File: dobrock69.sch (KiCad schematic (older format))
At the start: 159 parts, among them J1 HDMI_A_1.4, J2 Conn_01x02, J3 Conn_01x03, U1 XC6206P332MR, U2 STM32L072KBUx

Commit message: PCB switch daitai haichi shita
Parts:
- MX59, MX60, MX61, MX64, MX65, MX66: footprint kbd:CherryMX_Choc_Hotswap -> kbd:Choc_Hotswap
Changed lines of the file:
@@
 F 0 "MX60" H 3308 4298 60  0000 C CNN
 F 1 "MX-NoLED" H 3308 4224 20  0000 C CNN
-F 2 "kbd:CherryMX_Choc_Hotswap" H 2650 4050 60  0001 C CNN
+F 2 "kbd:Choc_Hotswap" H 2650 4050 60  0001 C CNN
 F 3 "" H 2650 4050 60  0001 C CNN
 	1    3275 4075
@@
 F 0 "MX59" H 2858 4298 60  0000 C CNN
 F 1 "MX-NoLED" H 2858 4224 20  0000 C CNN
-F 2 "kbd:CherryMX_Choc_Hotswap" H 2200 4050 60  0001 C CNN
+F 2 "kbd:Choc_Hotswap" H 2200 4050 60  0001 C CNN
 F 3 "" H 2200 4050 60  0001 C CNN
 	1    2825 4075
@@
 F 0 "MX61" H 3808 4298 60  0000 C CNN
 F 1 "MX-NoLED" H 3808 4224 20  0000 C CNN
-F 2 "kbd:CherryMX_Choc_Hotswap" H 3150 4050 60  0001 C CNN
+F 2 "kbd:Choc_Hotswap" H 3150 4050 60  0001 C CNN
 F 3 "" H 3150 4050 60  0001 C CNN
 	1    3775 4075
@@
 F 0 "MX64" H 9808 4373 60  0000 C CNN
 F 1 "MX-NoLED" H 9808 4299 20  0000 C CNN
-F 2 "kbd:CherryMX_Choc_Hotswap" H 9150 4125 60  0001 C CNN
+F 2 "kbd:Choc_Hotswap" H 9150 4125 60  0001 C CNN
 F 3 "" H 9150 4125 60  0001 C CNN
 	1    9775 4150
@@
 F 0 "MX66" H 10833 4373 60  0000 C CNN
 F 1 "MX-NoLED" H 10833 4299 20  0000 C CNN
-F 2 "kbd:CherryMX_Choc_Hotswap" H 10175 4125 60  0001 C CNN
+F 2 "kbd:Choc_Hotswap" H 10175 4125 60  0001 C CNN
 F 3 "" H 10175 4125 60  0001 C CNN
 	1    10800 4150
@@
 F 0 "MX65" H 10333 4373 60  0000 C CNN
 F 1 "MX-NoLED" H 10333 4299 20  0000 C CNN
-F 2 "kbd:CherryMX_Choc_Hotswap" H 9675 4125 60  0001 C CNN
+F 2 "kbd:Choc_Hotswap" H 9675 4125 60  0001 C CNN
 F 3 "" H 9675 4125 60  0001 C CNN
 	1    10300 4150

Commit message: pcb susunda
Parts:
- MX1, MX10, MX11, MX12, MX13, MX14, MX15, MX16, MX18, MX19, MX20, MX21, MX22, MX23, MX24, MX25, MX26, MX27, MX28, MX3, MX30, MX32, MX33, MX34, MX35, MX36, MX37, MX38, MX39, MX4, MX40, MX41, MX42, MX44, MX45, MX49, MX5, MX50, MX53, MX54, MX55, MX56, MX57, MX58, MX6, MX62, MX63, MX67, MX68, MX69, MX7, MX8, MX9: footprint MX_Only:MXOnly-1U-Hotswap -> MX_Only:MXOnly-1U-NoLED
- MX17, MX29: footprint MX_Only:MXOnly-1.75U-Hotswap -> MX_Only:MXOnly-1.75U-NoLED
- MX2: footprint MX_Only:MXOnly-1.5U-Hotswap -> MX_Only:MXOnly-1.5U-NoLED
- MX31, MX43, MX48, MX51: footprint MX_Only:MXOnly-2.25U-Hotswap -> MX_Only:MXOnly-2.25U-NoLED
- MX46, MX47, MX52: footprint MX_Only:MXOnly-1.25U-Hotswap -> MX_Only:MXOnly-1.25U-NoLED
- MX59, MX60, MX61, MX64, MX65, MX66: footprint kbd:Choc_Hotswap -> Kailh_Choc:KailhChoc-1U

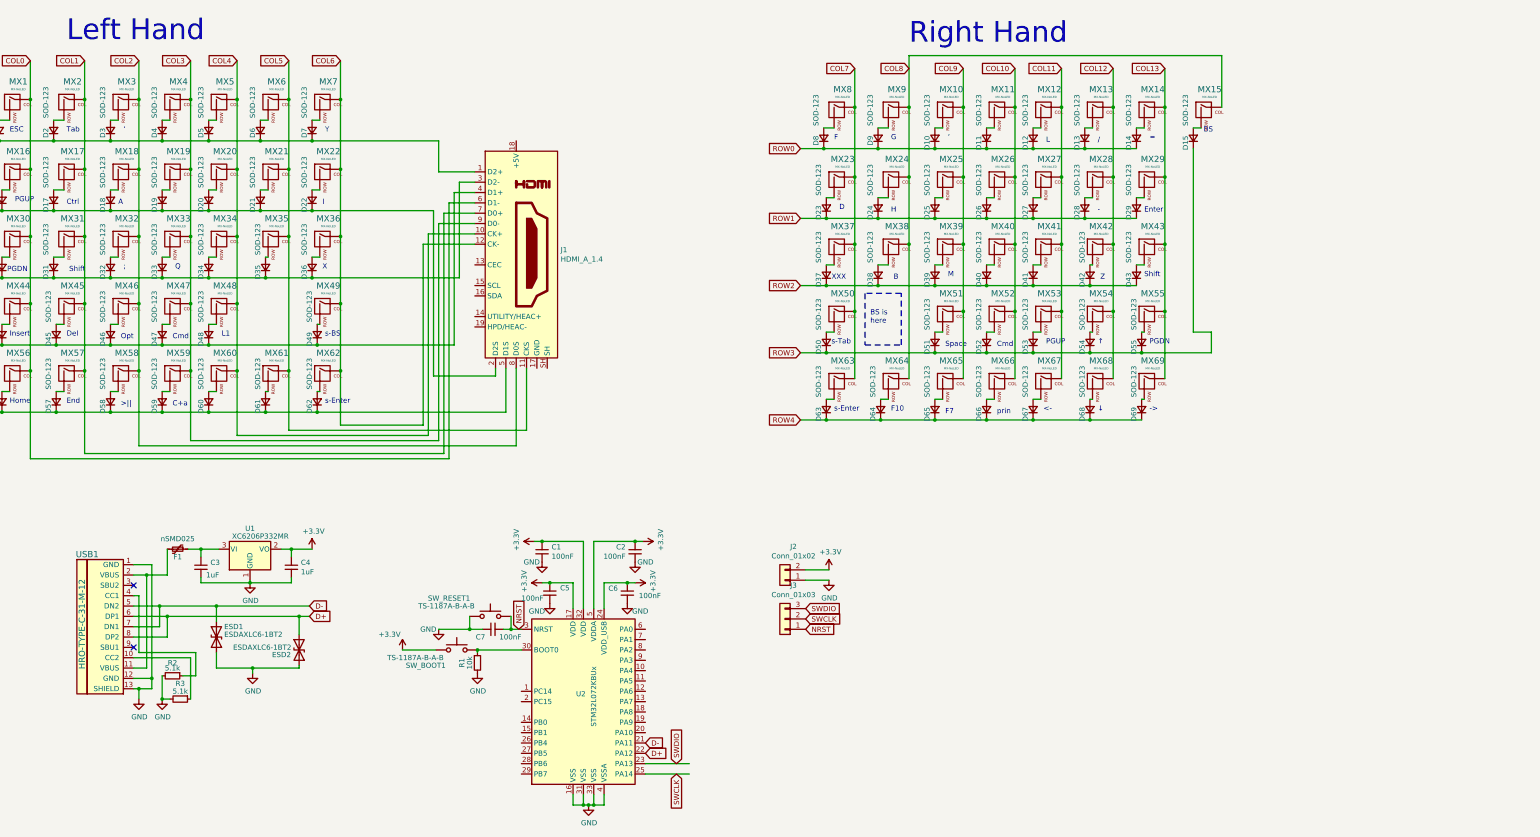
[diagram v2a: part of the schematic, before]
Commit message: pcb haisen susunda
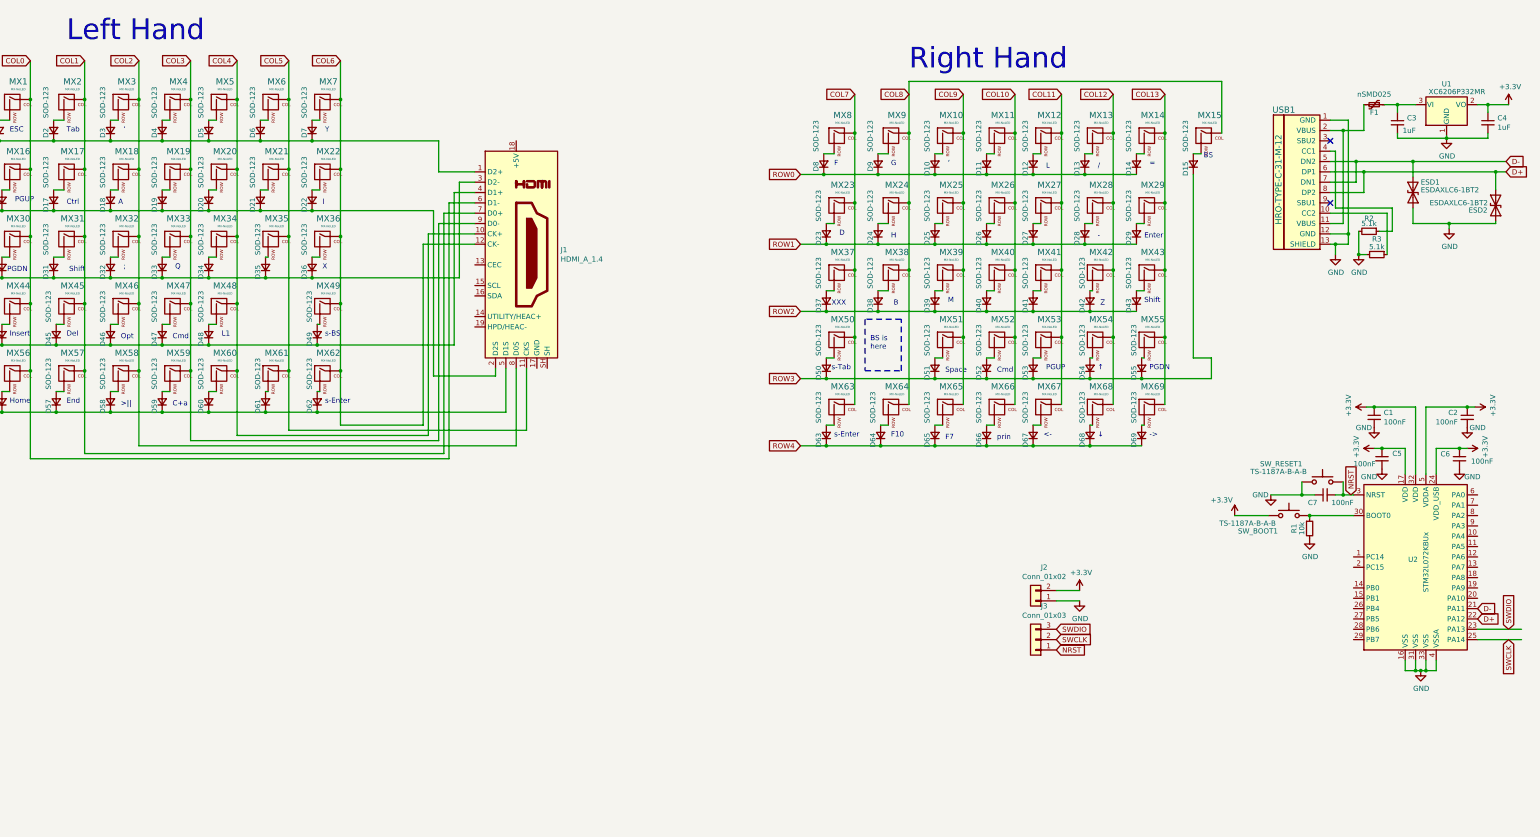
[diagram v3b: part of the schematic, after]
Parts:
- MX31, MX43, MX48, MX51: footprint MX_Only:MXOnly-2.25U-NoLED -> MX_Only:MXOnly-2.25U-ReversedStabilizers-NoLED
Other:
- moved on the sheet: C1, C2, C3, C4, C5, C6, C7, D10, D11, D12, D13, D14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
